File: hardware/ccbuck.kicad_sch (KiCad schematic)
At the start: 43 parts, among them J4 PWM/PFM, Q11 2N7002, Q7 2N7002, U1 TPS552872RYQR

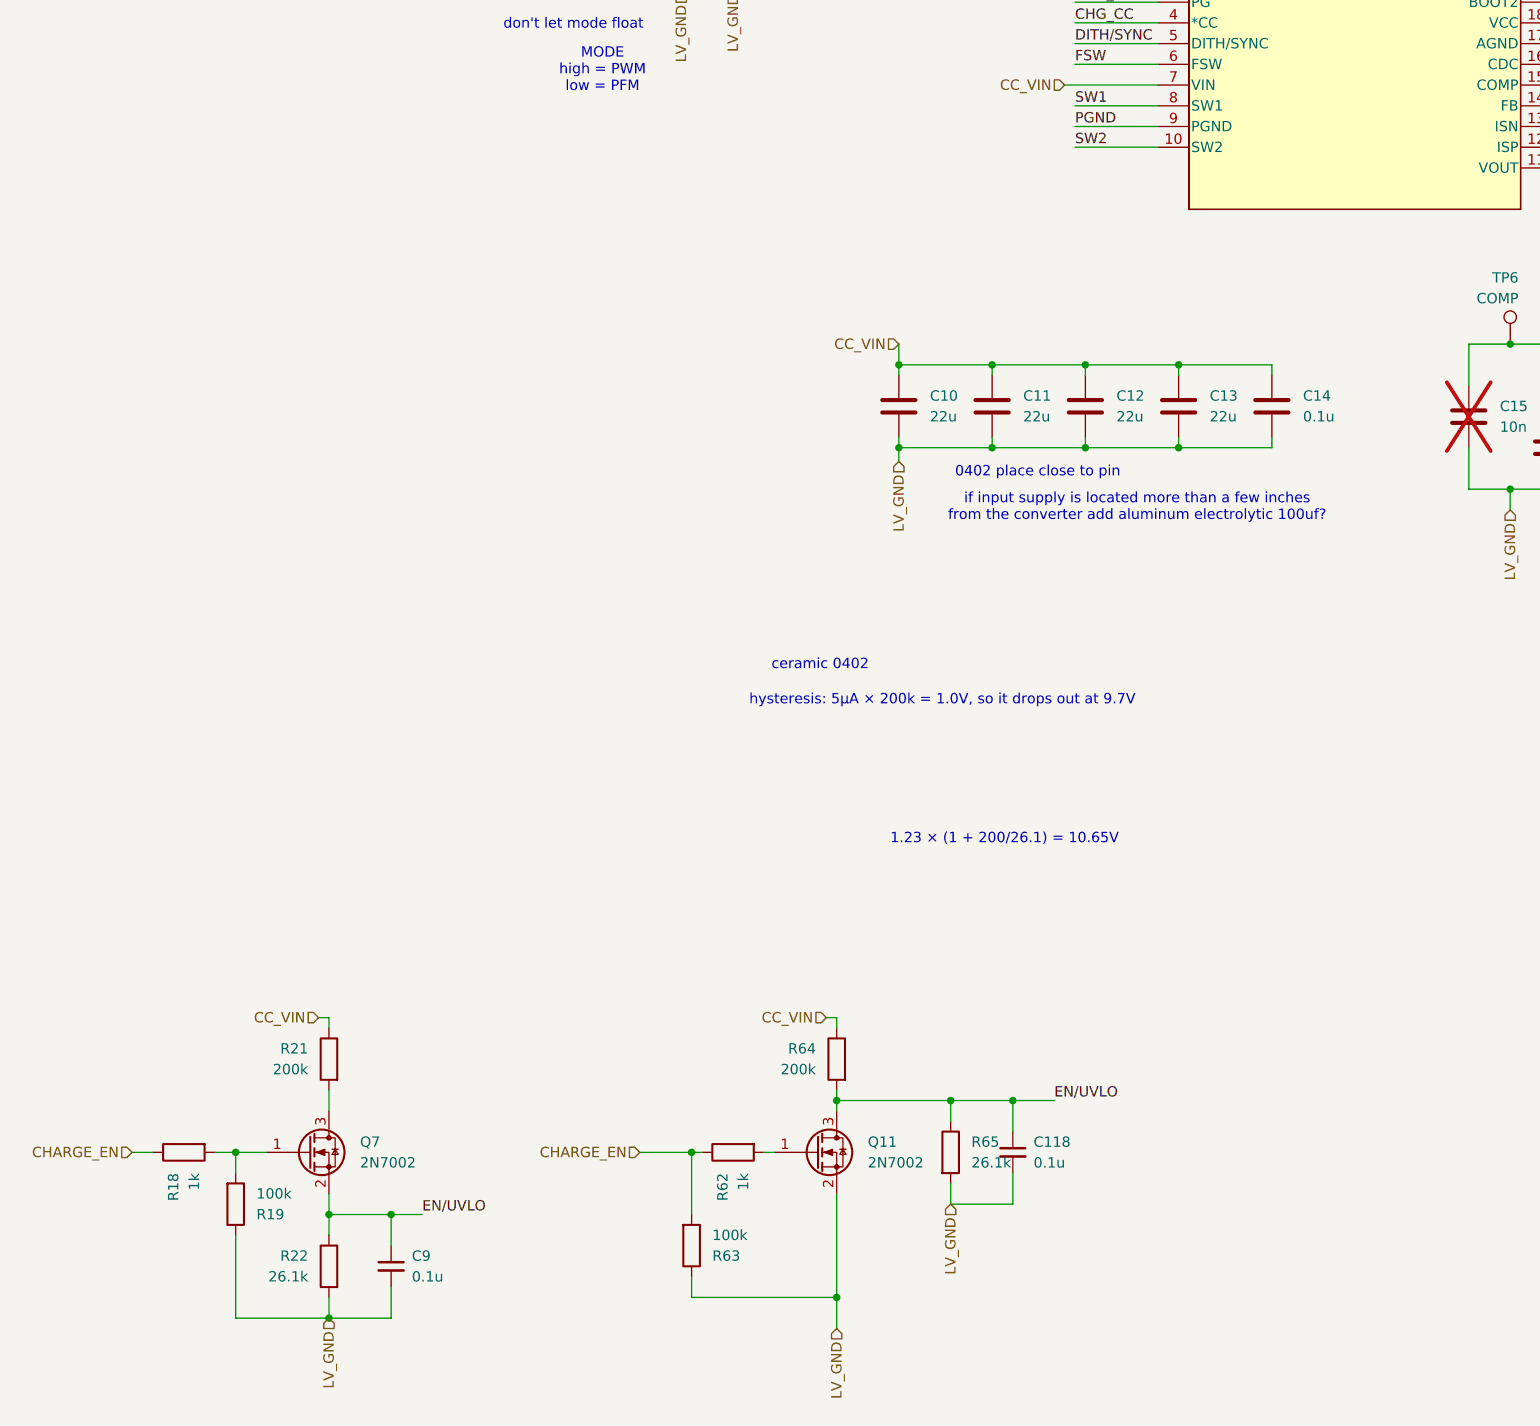
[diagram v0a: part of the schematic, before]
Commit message: switch back to pc
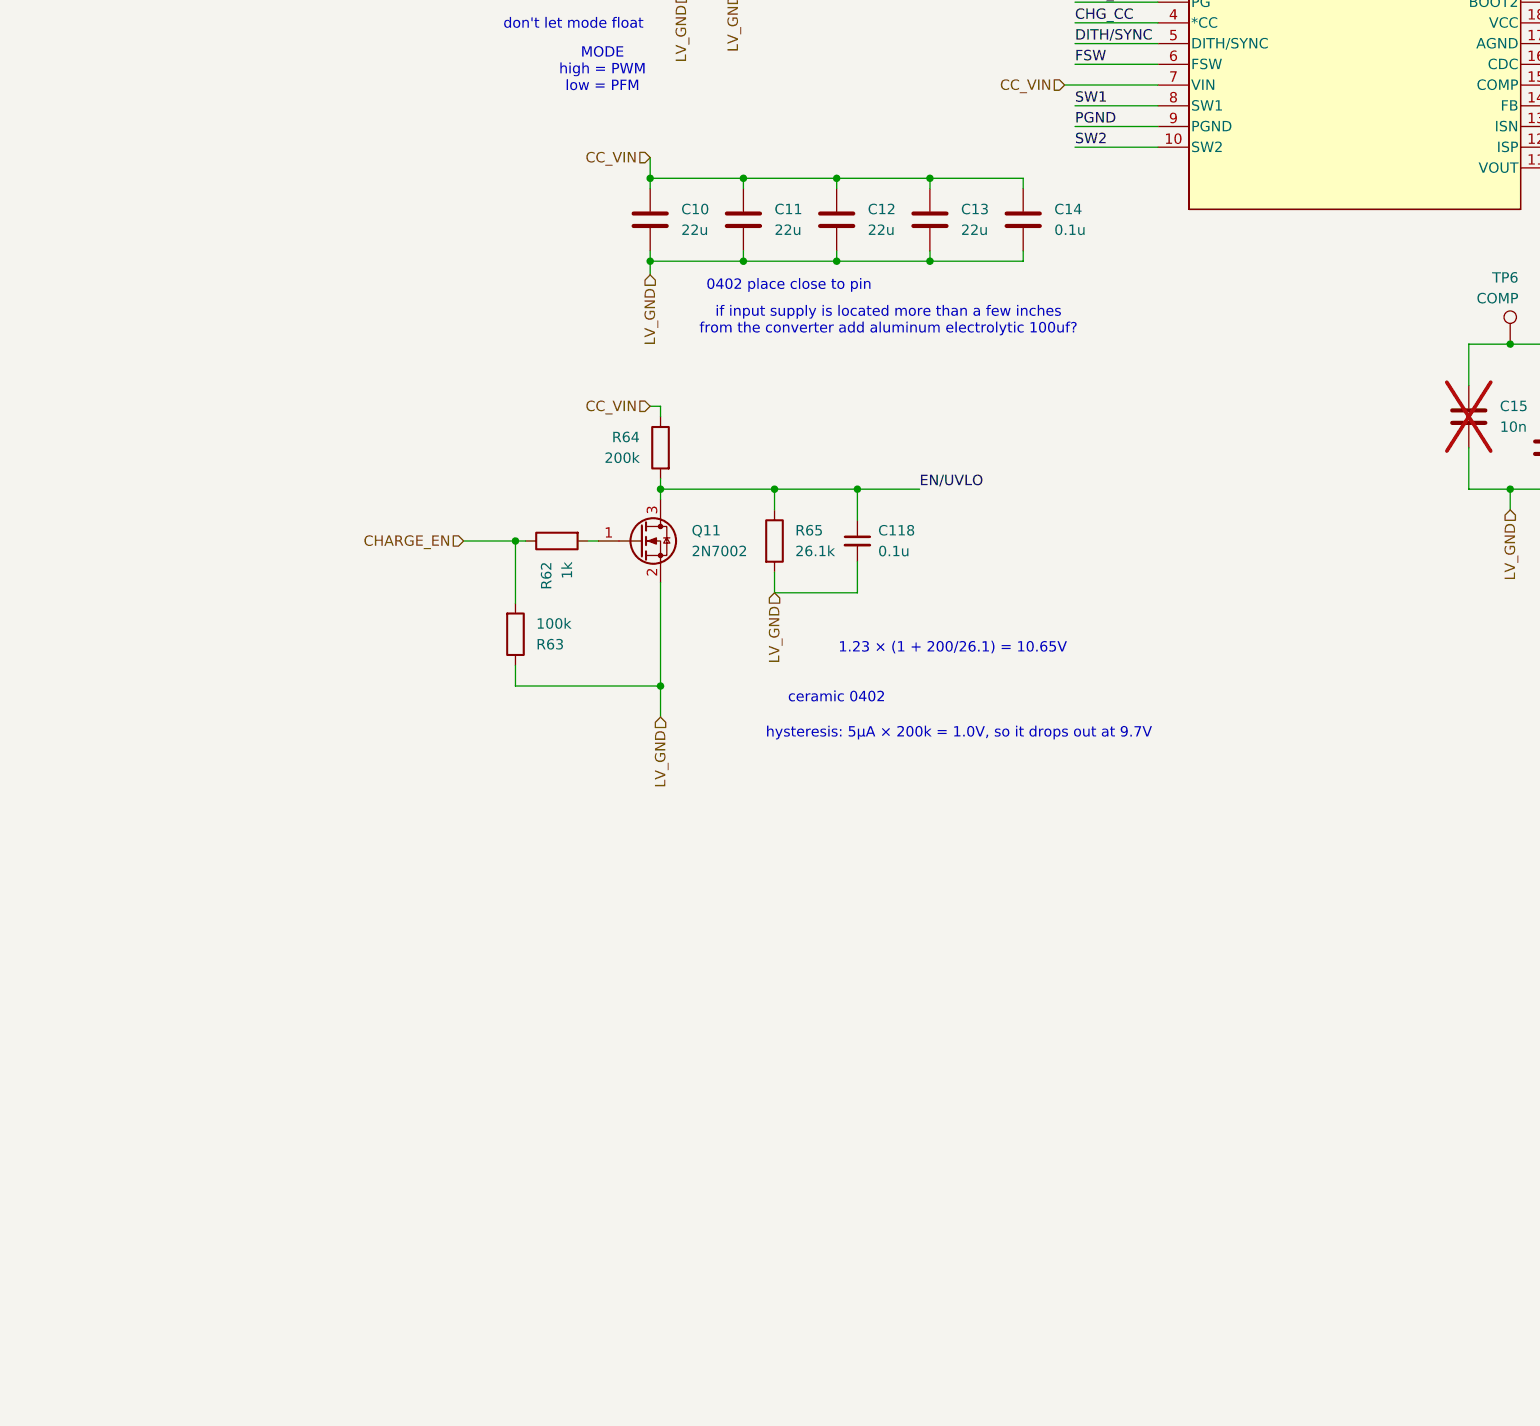
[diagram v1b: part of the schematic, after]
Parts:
- removed C9: 0.1u, Capacitor_SMD:C_0402_1005Metric_Pad0.74x0.62mm_HandSolder, symbol Device:C_Small
- removed Q7: 2N7002, Package_TO_SOT_SMD:SOT-23, symbol Transistor_FET:2N7002
- removed R18: 1k, Resistor_SMD:R_0603_1608Metric_Pad0.98x0.95mm_HandSolder, symbol Device:R
- removed R19: 100k, Resistor_SMD:R_0603_1608Metric_Pad0.98x0.95mm_HandSolder, symbol Device:R
- removed R21: 200k, Resistor_SMD:R_0603_1608Metric_Pad0.98x0.95mm_HandSolder, symbol Device:R
- removed R22: 26.1k, Resistor_SMD:R_0603_1608Metric_Pad0.98x0.95mm_HandSolder, symbol Device:R
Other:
- moved on the sheet: C10, C11, C118, C12, C13, C14, Q11, R62, R63, R64, R65
